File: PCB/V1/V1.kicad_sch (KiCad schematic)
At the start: 17 parts, among them J1 Bornera Motores, J2 Bateria2, J3 Bateria1, SW1 SW ON/OFF MOTORES, SW2 SW 24V/12V, SW3 SW ON/OFF, U1 ESP32-Devkit-V1

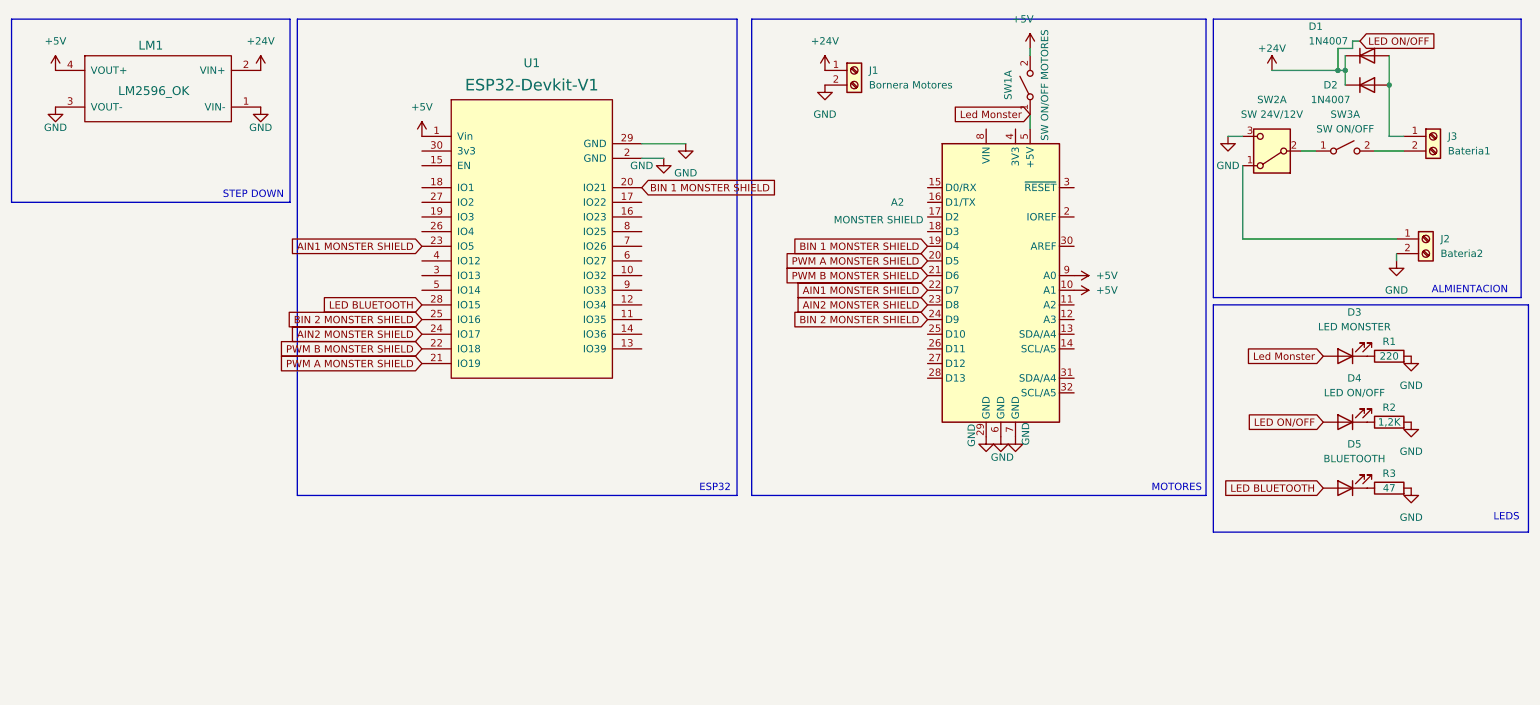
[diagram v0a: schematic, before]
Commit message: .
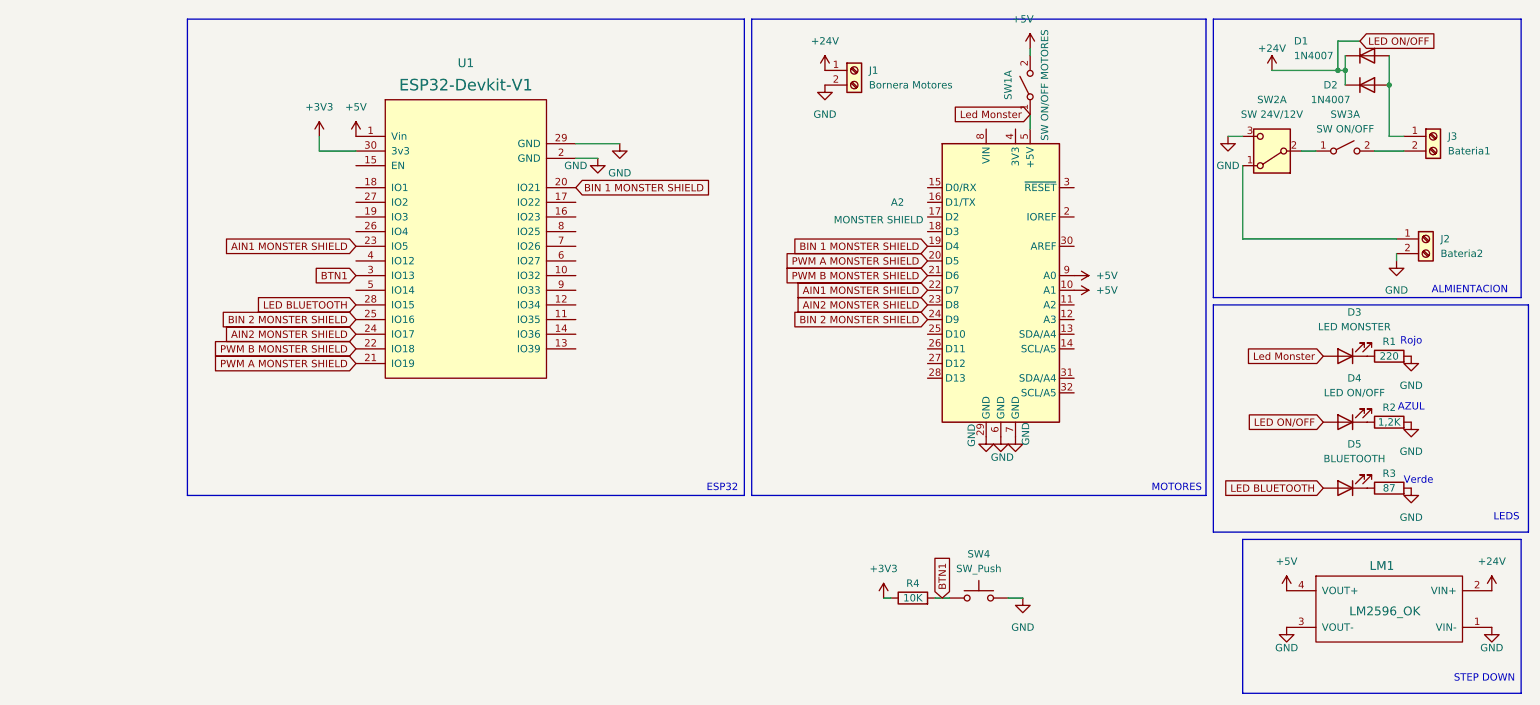
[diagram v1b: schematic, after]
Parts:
- added R4: 10K, Resistor_THT:R_Axial_DIN0207_L6.3mm_D2.5mm_P10.16mm_Horizontal, symbol Device:R
- added SW4: SW_Push, TerminalBlock:TerminalBlock_bornier-2_P5.08mm, symbol Switch:SW_Push
- D5: footprint LED_THT:LED_D5.0mm_Horizontal_O1.27mm_Z3.0mm -> Connector_Molex:Molex_KK-254_AE-6410-02A_1x02_P2.54mm_Vertical
- R3: value 47 -> 87
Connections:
- net GND: now also SW4.2
- net BTN1: now reaches U1.3 (IO13)
- net BTN1: now also R4.2, SW4.1
- net +3V3: now reaches U1.30 (3v3)
- net +3V3: now also R4.1
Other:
- note added: "AZUL"
- note added: "Rojo"
- note added: "Verde"
- moved on the sheet: LM1, U1
